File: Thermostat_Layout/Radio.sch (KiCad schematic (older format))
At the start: 1 part, among them U10 ESP-07

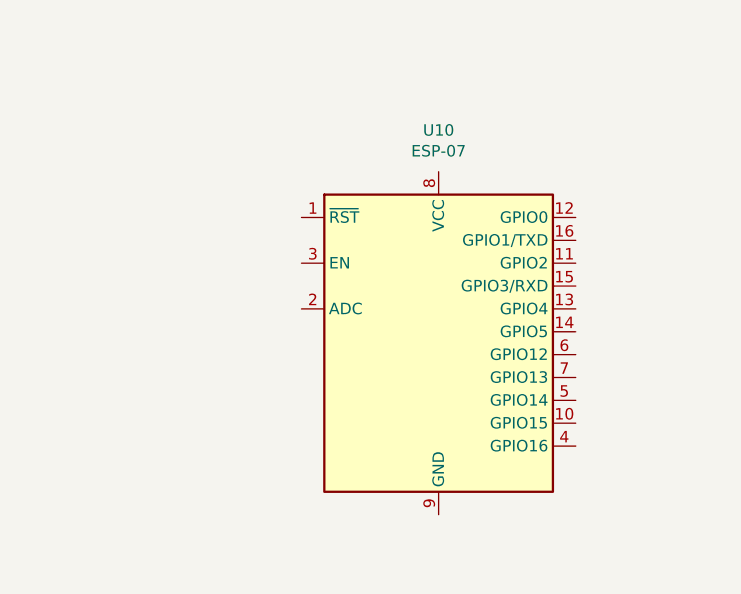
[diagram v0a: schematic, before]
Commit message: Layout changes
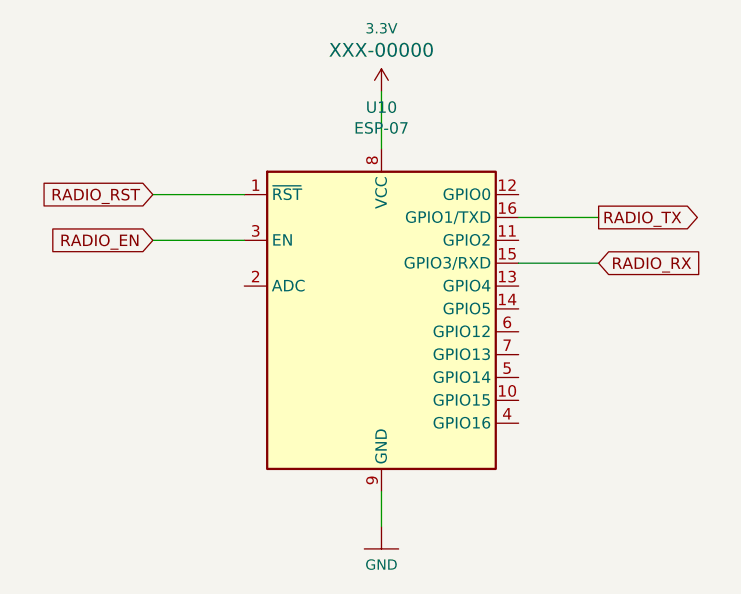
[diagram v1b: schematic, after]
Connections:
- net RADIO_RST: now reaches U10.1 (~RST)
- net RADIO_RX: now reaches U10.15 (GPIO3/RXD)
- net RADIO_TX: now reaches U10.16 (GPIO1/TXD)
- net RADIO_EN: now reaches U10.3 (EN)
- net 3.3V: now reaches U10.8 (VCC)
- net GND: now reaches U10.9 (GND)
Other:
- moved on the sheet: U10
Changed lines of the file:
@@
 L RF_Module:ESP-07 U10
 U 1 1 5D98C19F
-P 5900 3650
-F 0 "U10" H 5900 4631 50  0000 C CNN
-F 1 "ESP-07" H 5900 4540 50  0000 C CNN
-F 2 "RF_Module:ESP-07" H 5900 3650 50  0001 C CNN
-F 3 "http://wiki.ai-thinker.com/_media/esp8266/esp8266_series_modules_user_manual_v1.1.pdf" H 5550 3750 50  0001 C CNN
-	1    5900 3650
+P 5650 3550
+F 0 "U10" H 5650 4531 50  0000 C CNN
+F 1 "ESP-07" H 5650 4440 50  0000 C CNN
+F 2 "RF_Module:ESP-07" H 5650 3550 50  0001 C CNN
+F 3 "http://wiki.ai-thinker.com/_media/esp8266/esp8266_series_modules_user_manual_v1.1.pdf" H 5300 3650 50  0001 C CNN
+	1    5650 3550
 	1    0    0    -1
 $EndComp
+Text GLabel 6600 3050 2    50   Output ~ 0
+RADIO_TX
+Text GLabel 6600 3250 2    50   Input ~ 0
+RADIO_RX
+Wire Wire Line
+	6250 3050 6600 3050
+Wire Wire Line
+	6250 3250 6600 3250
+$Comp
+L SparkFun-PowerSymbols:3.3V #SUPPLY?
+U 1 1 5D9E7A19
+P 5650 2500
+F 0 "#SUPPLY?" H 5700 2500 45  0001 L BNN
+F 1 "3.3V" H 5650 2776 45  0000 C CNN
+F 2 "XXX-00000" H 5650 2681 60  0000 C CNN
+F 3 "" H 5650 2500 60  0001 C CNN
+	1    5650 2500
+	1    0    0    -1
+$EndComp
+$Comp
+L SparkFun-PowerSymbols:GND #GND?
+U 1 1 5D9E8201
+P 5650 4400
+F 0 "#GND?" H 5700 4350 45  0001 L BNN
+F 1 "GND" H 5650 4230 45  0000 C CNN
+F 2 "" H 5650 4300 60  0001 C CNN
+F 3 "" H 5650 4300 60  0001 C CNN
+	1    5650 4400
+	1    0    0    -1
+$EndComp
+Wire Wire Line
+	5650 4250 5650 4400
+Wire Wire Line
+	5650 2750 5650 2500
+Text GLabel 4650 2950 0    50   Input ~ 0
+RADIO_RST
+Text GLabel 4650 3150 0    50   Input ~ 0
+RADIO_EN
+Wire Wire Line
+	4650 2950 5050 2950
+Wire Wire Line
+	5050 3150 4650 3150
 $EndSCHEMATC
